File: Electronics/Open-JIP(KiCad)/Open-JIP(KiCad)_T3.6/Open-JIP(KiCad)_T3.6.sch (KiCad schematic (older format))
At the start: 31 parts, among them J1 EJ503A, J2 Screw_Terminal_01x02, U1 74HC4066D,653, U2 74HC4066D,653, U3 KA7812ETU, U4 OPA320AIDBVT, U5 Teensy3.6

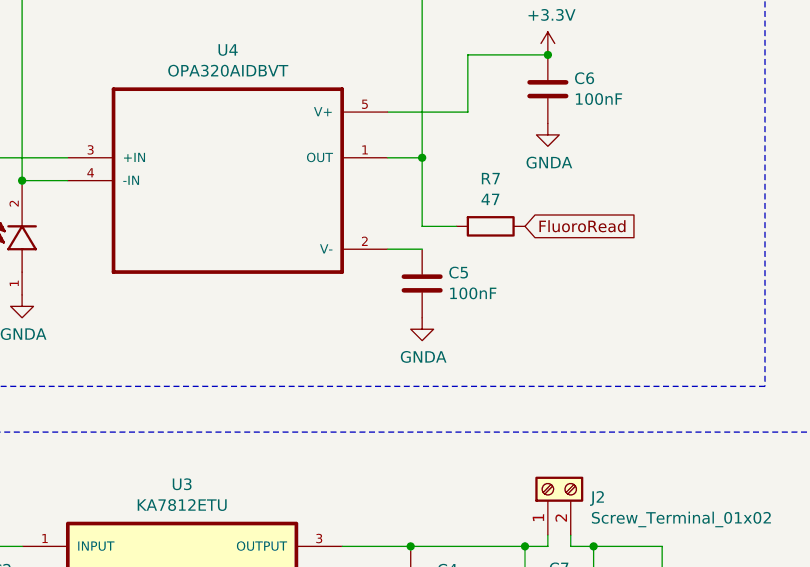
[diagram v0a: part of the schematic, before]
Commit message: finished v0.3 for teensy 3.2 and added gerber files
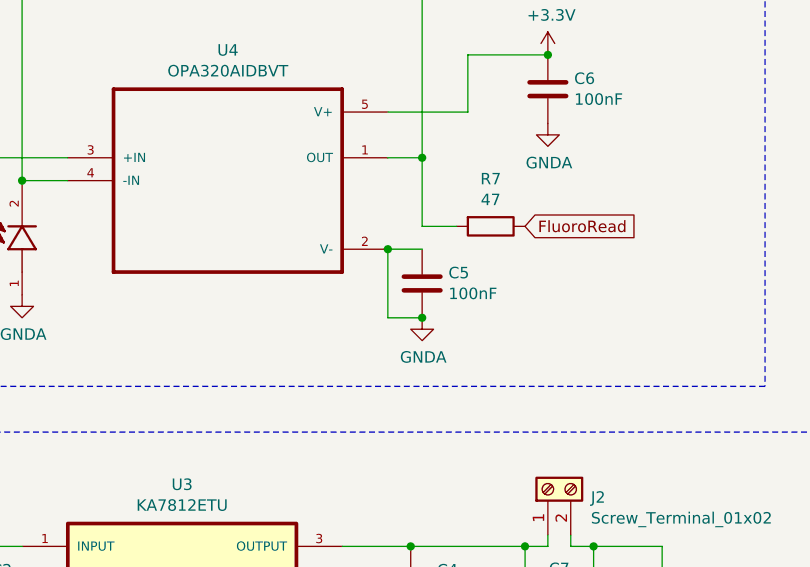
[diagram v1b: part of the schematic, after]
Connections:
- net GNDA: now also C5.2, U4.2 (V-)
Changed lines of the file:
@@
 	1950 5250 1950 5350
 Connection ~ 1950 5350
+Wire Wire Line
+	4300 3800 4300 4100
+Wire Wire Line
+	4300 4100 4450 4100
+Connection ~ 4300 3800
+Connection ~ 4450 4100
 $EndSCHEMATC
